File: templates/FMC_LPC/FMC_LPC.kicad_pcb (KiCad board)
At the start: 4 copper layers, 76.5 x 69 mm, 42 parts, among them CN1 FMC_Mezzanine, M1 Logo_10mmx10mm, U1 24LC02BT-I/MNY, U2 LM73100RPWR, U3 LM73100RPWR, U4 LM73100RPWR

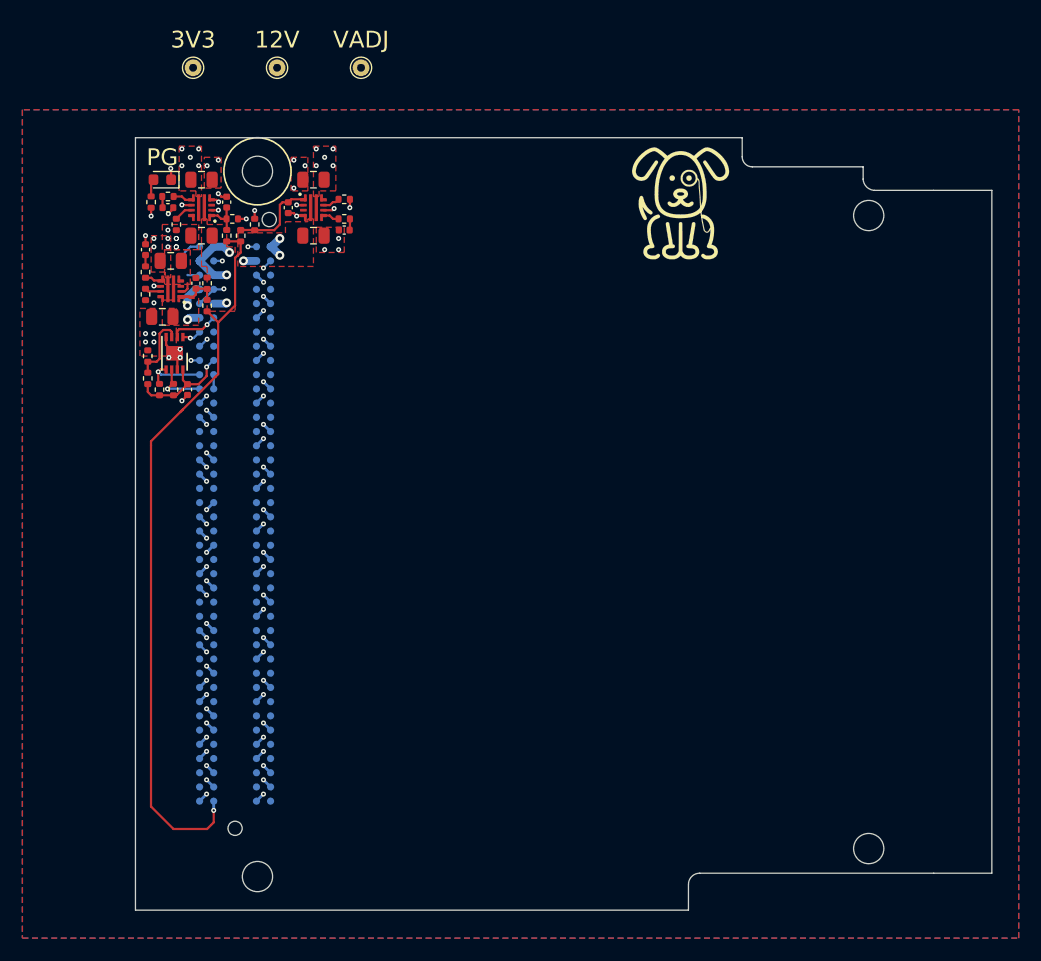
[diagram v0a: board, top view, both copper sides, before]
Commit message: New system actually works now
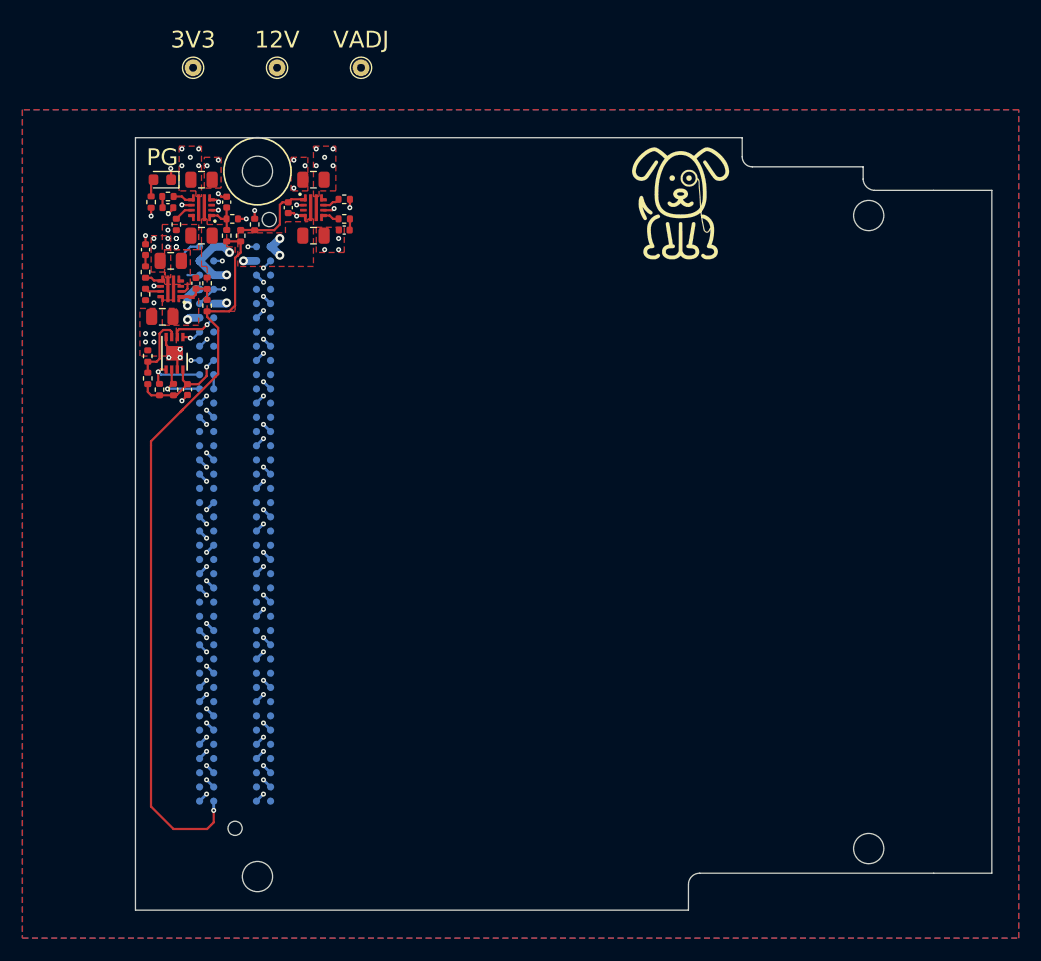
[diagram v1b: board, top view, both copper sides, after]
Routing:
- net /FMC Connector/PG_C2M: track 65.3 -> 65.9 mm
